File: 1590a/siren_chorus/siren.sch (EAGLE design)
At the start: 52 parts, among them IC1 NE5532, Q1 2N5457

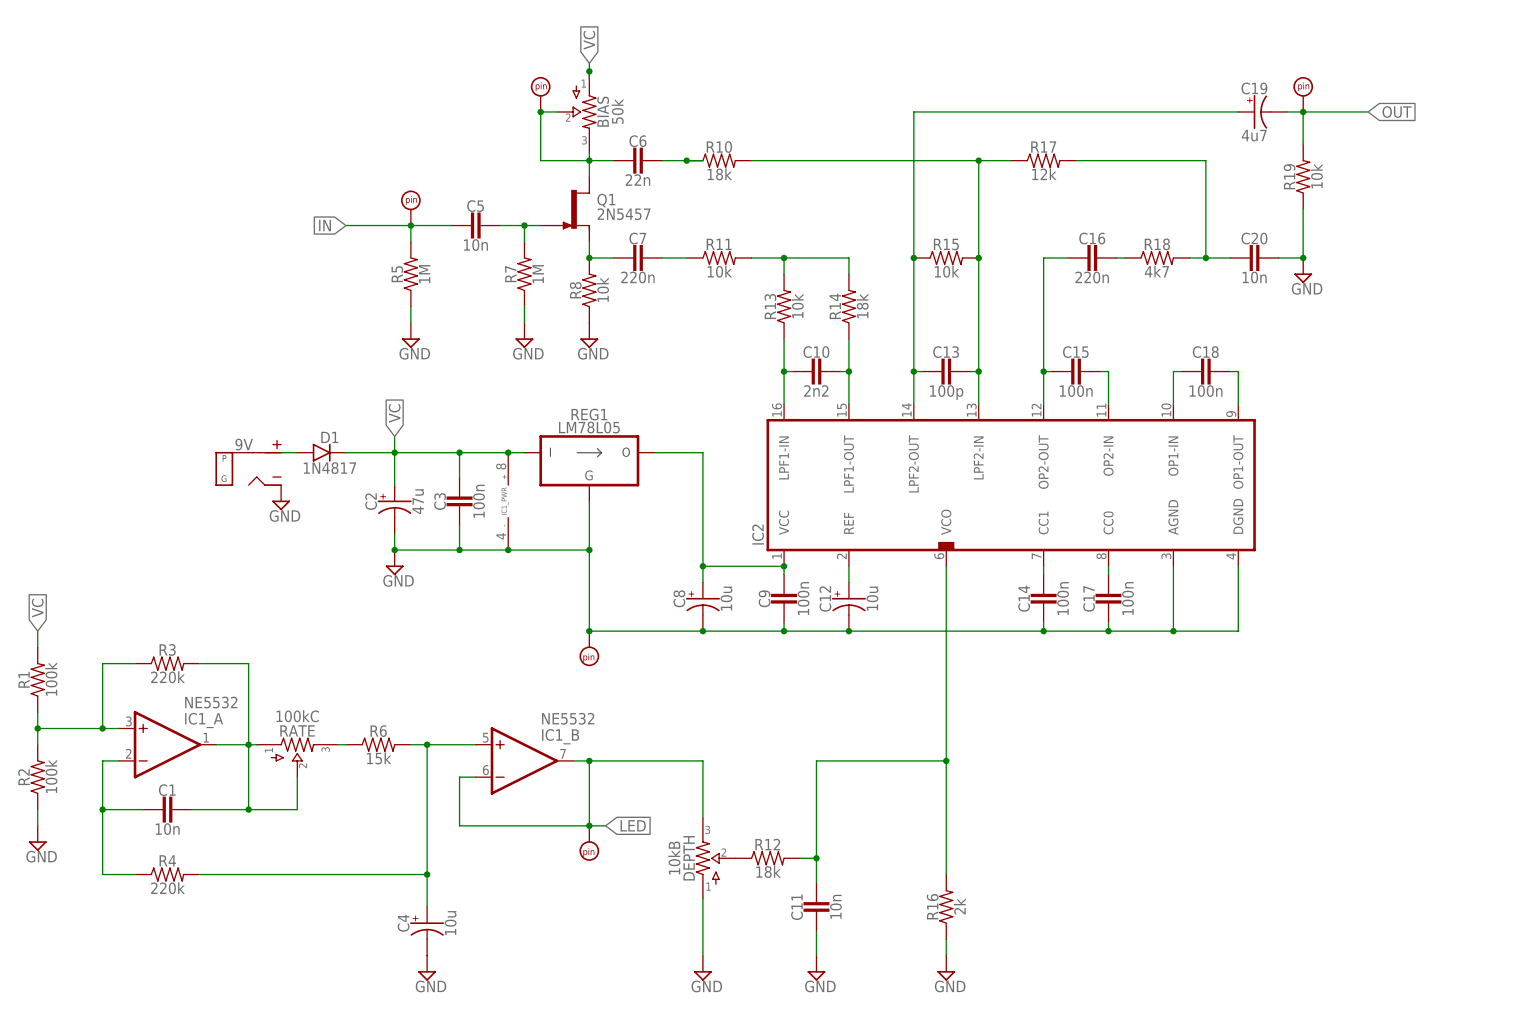
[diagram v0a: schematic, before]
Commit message: finished chorus and tremolo baords; other tweaks & polish
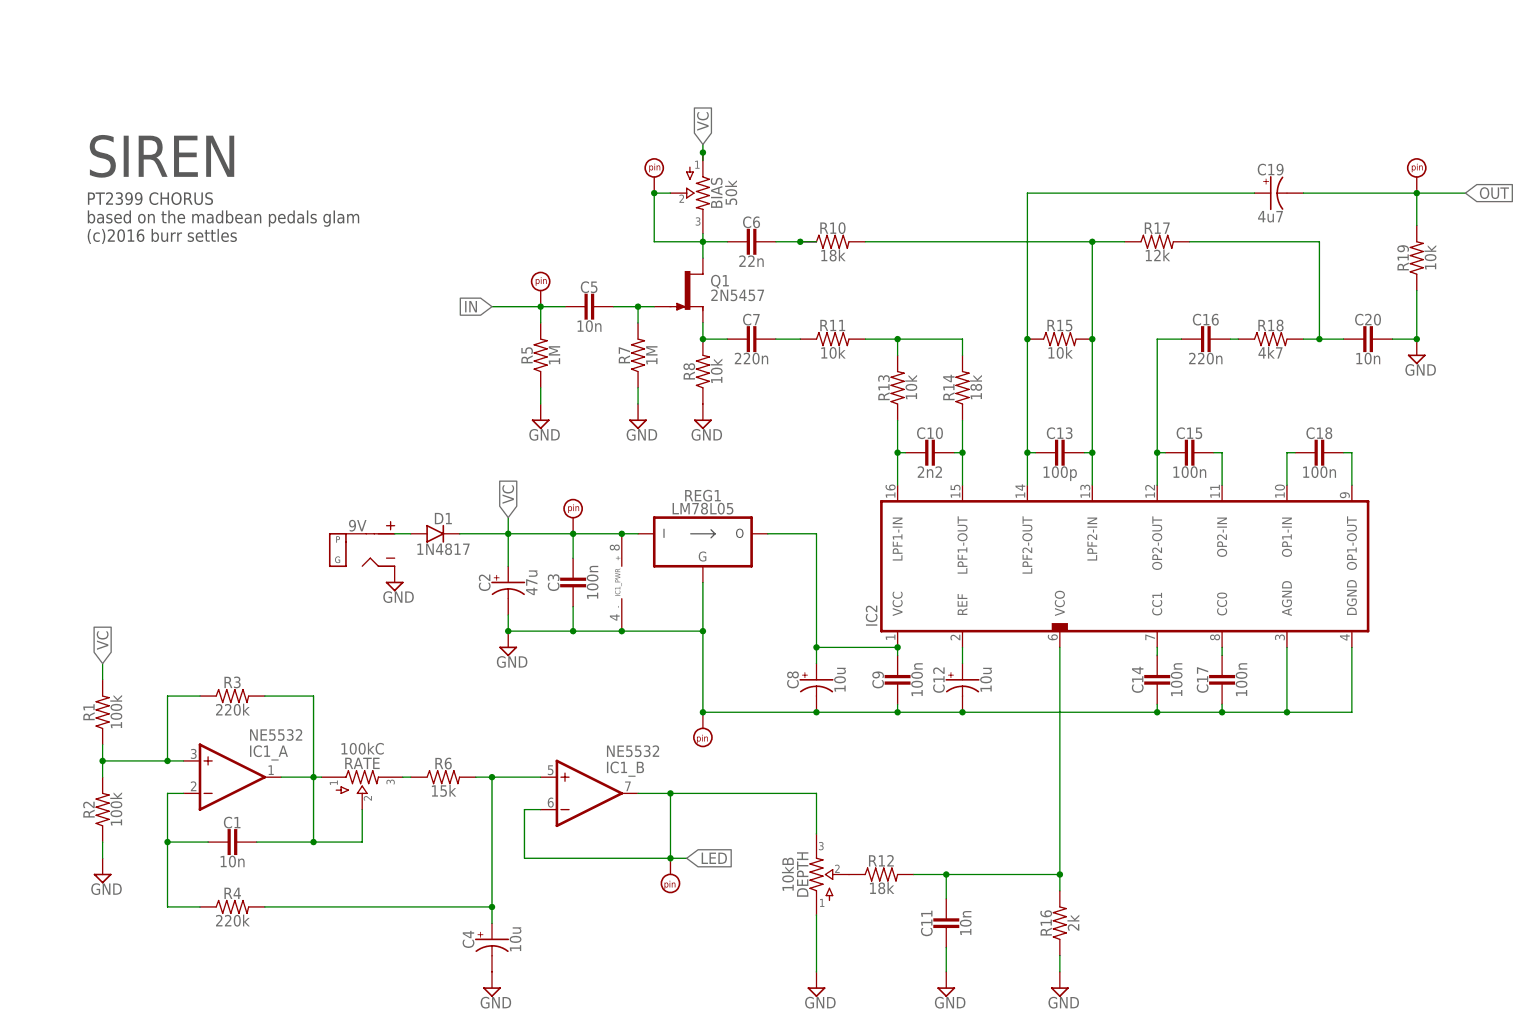
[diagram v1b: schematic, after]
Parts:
- removed LED: PADSQR, supply pins:PADSQR
- added L+: PADSQR, supply pins:PADSQR
- added PAD1: PAD, supply pins:PAD
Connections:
- net LED: now also L+.P$1; no longer LED.P$1
- net VC: now also PAD1.P$1
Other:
- note added: "PT2399 CHORUS based on the madbean pedals glam (c)2016 burr settles"
- note added: "SIREN"
- moved on the sheet: 9V, BIAS, C1, C10, C11, C12, C13, C14, C15, C16, C17, C18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
